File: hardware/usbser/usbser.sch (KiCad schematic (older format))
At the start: 18 parts, among them J2 STM32WORLD_BASE, U1 XC6206P332MR, U2 CP2102N

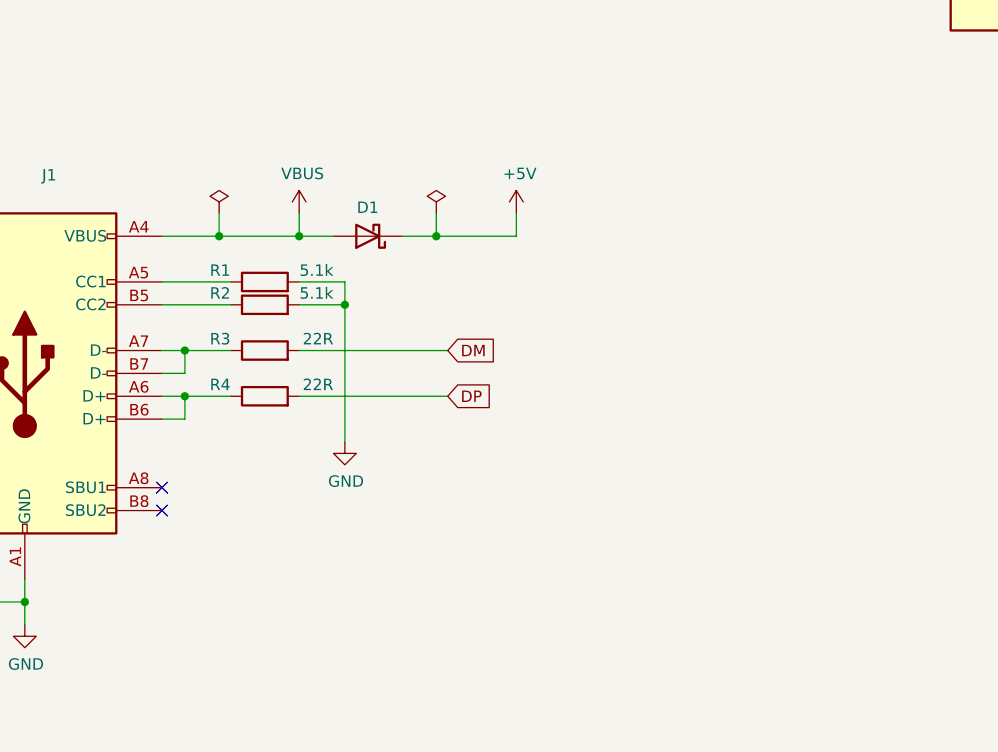
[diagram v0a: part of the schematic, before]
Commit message: Hmmmm
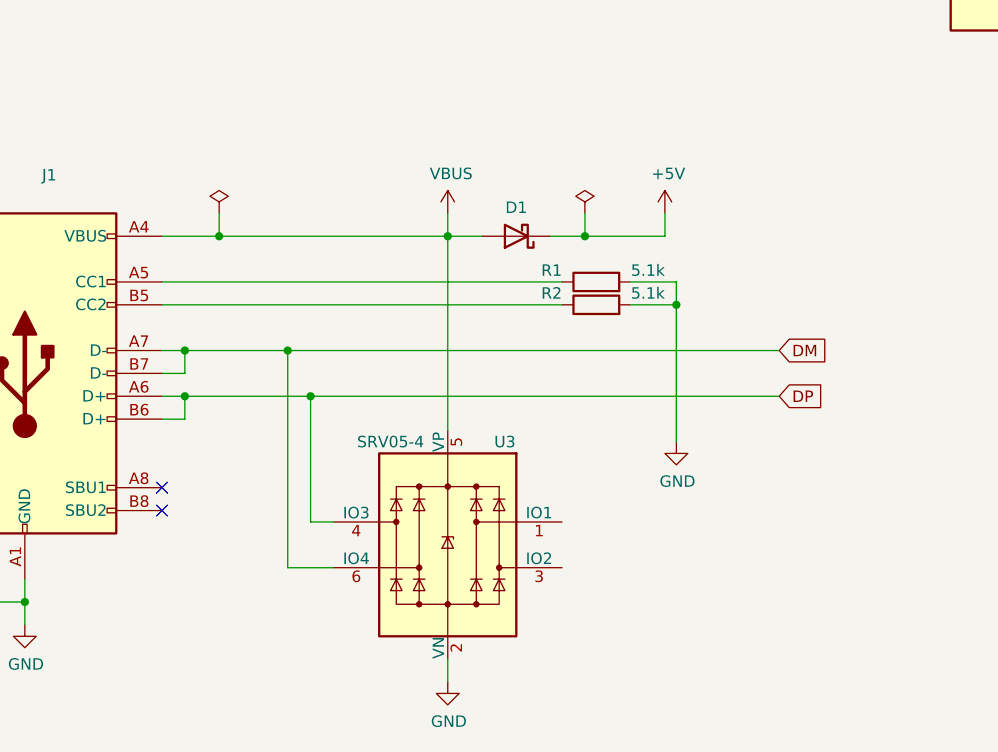
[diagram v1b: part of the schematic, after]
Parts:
- removed R3, R4: 22R, Resistor_SMD:R_0402_1005Metric, symbol Device:R
- added U3: SRV05-4, Package_TO_SOT_SMD:SOT-23-6, symbol Power_Protection:SRV05-4
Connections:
- net DM: now also J1.A7 (D-), J1.B7 (D-), U3.6 (IO4)
- net DP: now also J1.A6 (D+), J1.B6 (D+), U3.4 (IO3)
- net GND: now also U3.2 (VN)
- net VBUS: now also U3.5 (VP)
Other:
- moved on the sheet: D1, R1, R2
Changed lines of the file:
@@
 L Device:D_Schottky D?
 U 1 1 61254E07
-P 2800 5500
+P 3450 5500
 AR Path="/60D07374/61254E07" Ref="D?"  Part="1"
 AR Path="/61254E07" Ref="D1"  Part="1"
-F 0 "D1" H 2800 5375 50  0000 C CNN
-F 1 "~" H 2800 5374 50  0000 C CNN
-F 2 "Diode_SMD:D_SOD-123" H 2800 5500 50  0001 C CNN
-F 3 "~" H 2800 5500 50  0001 C CNN
-F 4 "C8598" H 2800 5500 50  0001 C CNN "LCSC"
-	1    2800 5500
+F 0 "D1" H 3450 5375 50  0000 C CNN
+F 1 "~" H 3450 5374 50  0000 C CNN
+F 2 "Diode_SMD:D_SOD-123" H 3450 5500 50  0001 C CNN
+F 3 "~" H 3450 5500 50  0001 C CNN
+F 4 "C8598" H 3450 5500 50  0001 C CNN "LCSC"
+	1    3450 5500
 	-1   0    0    1
 $EndComp
@@
 Wire Wire Line
 	1900 6000 2000 6000
-Text GLabel 3150 6200 2    50   Input ~ 0
+Text GLabel 4600 6200 2    50   Input ~ 0
 DP
-Text GLabel 3150 6000 2    50   Input ~ 0
+Text GLabel 4600 6000 2    50   Input ~ 0
 DM
 $Comp
 L Device:R R?
 U 1 1 61254E17
-P 2350 5700
+P 3800 5700
 AR Path="/60D07374/61254E17" Ref="R?"  Part="1"
 AR Path="/61254E17" Ref="R1"  Part="1"
-F 0 "R1" V 2400 5850 50  0000 L CNN
-F 1 "5.1k" V 2400 5400 50  0000 L CNN
-F 2 "Resistor_SMD:R_0402_1005Metric" V 2280 5700 50  0001 C CNN
-F 3 "~" H 2350 5700 50  0001 C CNN
-F 4 "C25905" H 2350 5700 50  0001 C CNN "LCSC"
-	1    2350 5700
+F 0 "R1" V 3850 5850 50  0000 L CNN
+F 1 "5.1k" V 3850 5400 50  0000 L CNN
+F 2 "Resistor_SMD:R_0402_1005Metric" V 3730 5700 50  0001 C CNN
+F 3 "~" H 3800 5700 50  0001 C CNN
+F 4 "C25905" H 3800 5700 50  0001 C CNN "LCSC"
+	1    3800 5700
 	0    -1   -1   0
 $EndComp
@@
 L Device:R R?
 U 1 1 61254E2C
-P 2350 5800
+P 3800 5800
 AR Path="/60D07374/61254E2C" Ref="R?"  Part="1"
 AR Path="/61254E2C" Ref="R2"  Part="1"
-F 0 "R2" V 2400 5950 50  0000 L CNN
-F 1 "5.1k" V 2400 5500 50  0000 L CNN
-F 2 "Resistor_SMD:R_0402_1005Metric" V 2280 5800 50  0001 C CNN
-F 3 "~" H 2350 5800 50  0001 C CNN
-F 4 "C25905" H 2350 5800 50  0001 C CNN "LCSC"
-	1    2350 5800
+F 0 "R2" V 3850 5950 50  0000 L CNN
+F 1 "5.1k" V 3850 5500 50  0000 L CNN
+F 2 "Resistor_SMD:R_0402_1005Metric" V 3730 5800 50  0001 C CNN
+F 3 "~" H 3800 5800 50  0001 C CNN
+F 4 "C25905" H 3800 5800 50  0001 C CNN "LCSC"
+	1    3800 5800
 	0    -1   -1   0
 $EndComp
@@
 L power:VBUS #PWR?
 U 1 1 61254E38
-P 2500 5400
+P 3150 5400
 AR Path="/60D07374/61254E38" Ref="#PWR?"  Part="1"
 AR Path="/61254E38" Ref="#PWR0102"  Part="1"
-F 0 "#PWR0102" H 2500 5250 50  0001 C CNN
-F 1 "VBUS" H 2515 5573 50  0000 C CNN
-F 2 "" H 2500 5400 50  0001 C CNN
-F 3 "" H 2500 5400 50  0001 C CNN
-	1    2500 5400
-	1    0    0    -1
-$EndComp
-Wire Wire Line
-	2950 5500 3100 5500
-Wire Wire Line
-	3450 5500 3450 5400
+F 0 "#PWR0102" H 3150 5250 50  0001 C CNN
+F 1 "VBUS" H 3165 5573 50  0000 C CNN
+F 2 "" H 3150 5400 50  0001 C CNN
+F 3 "" H 3150 5400 50  0001 C CNN
+	1    3150 5400
+	1    0    0    -1
+$EndComp
+Wire Wire Line
+	3600 5500 3750 5500
+Wire Wire Line
+	4100 5500 4100 5400
 $Comp
 L power:+5V #PWR?
 U 1 1 61254E40
-P 3450 5400
+P 4100 5400
 AR Path="/60D07374/61254E40" Ref="#PWR?"  Part="1"
 AR Path="/61254E40" Ref="#PWR0103"  Part="1"
-F 0 "#PWR0103" H 3450 5250 50  0001 C CNN
-F 1 "+5V" H 3465 5573 50  0000 C CNN
-F 2 "" H 3450 5400 50  0001 C CNN
-F 3 "" H 3450 5400 50  0001 C CNN
-	1    3450 5400
-	1    0    0    -1
-$EndComp
-Wire Wire Line
-	2500 5400 2500 5500
-Connection ~ 2500 5500
-Wire Wire Line
-	2500 5500 2650 5500
-$Comp
-L Device:R R?
-U 1 1 61254E4A
-P 2350 6000
-AR Path="/60D07374/61254E4A" Ref="R?"  Part="1"
-AR Path="/61254E4A" Ref="R3"  Part="1"
-F 0 "R3" V 2400 6150 50  0000 L CNN
-F 1 "22R" V 2400 5700 50  0000 L CNN
-F 2 "Resistor_SMD:R_0402_1005Metric" V 2280 6000 50  0001 C CNN
-F 3 "~" H 2350 6000 50  0001 C CNN
-F 4 "C25092" H 2350 6000 50  0001 C CNN "LCSC"
-	1    2350 6000
-	0    -1   -1   0
-$EndComp
-$Comp
-L Device:R R?
-U 1 1 61254E51
-P 2350 6200
-AR Path="/60D07374/61254E51" Ref="R?"  Part="1"
-AR Path="/61254E51" Ref="R4"  Part="1"
-F 0 "R4" V 2400 6350 50  0000 L CNN
-F 1 "22R" V 2400 5900 50  0000 L CNN
-F 2 "Resistor_SMD:R_0402_1005Metric" V 2280 6200 50  0001 C CNN
-F 3 "~" H 2350 6200 50  0001 C CNN
-F 4 "C25092" H 2350 6200 50  0001 C CNN "LCSC"
-	1    2350 6200
-	0    -1   -1   0
-$EndComp
-Wire Wire Line
-	3150 6000 2500 6000
-Wire Wire Line
-	3150 6200 2500 6200
-Wire Wire Line
-	2000 6200 2200 6200
-Wire Wire Line
-	2000 6000 2200 6000
+F 0 "#PWR0103" H 4100 5250 50  0001 C CNN
+F 1 "+5V" H 4115 5573 50  0000 C CNN
+F 2 "" H 4100 5400 50  0001 C CNN
+F 3 "" H 4100 5400 50  0001 C CNN
+	1    4100 5400
+	1    0    0    -1
+$EndComp
+Wire Wire Line
+	3150 5400 3150 5500
+Connection ~ 3150 5500
+Wire Wire Line
+	3150 5500 3300 5500
 $Comp
 L power:PWR_FLAG #FLG?
@@
 Connection ~ 2150 5500
 Wire Wire Line
-	2150 5500 2500 5500
+	2150 5500 3150 5500
 NoConn ~ 1900 6600
 NoConn ~ 1900 6700
@@
 L power:PWR_FLAG #FLG?
 U 1 1 61254E66
-P 3100 5400
+P 3750 5400
 AR Path="/60D07374/61254E66" Ref="#FLG?"  Part="1"
 AR Path="/61254E66" Ref="#FLG0102"  Part="1"
-F 0 "#FLG0102" H 3100 5475 50  0001 C CNN
-F 1 "PWR_FLAG" H 3100 5573 50  0001 C CNN
-F 2 "" H 3100 5400 50  0001 C CNN
-F 3 "~" H 3100 5400 50  0001 C CNN
-	1    3100 5400
-	1    0    0    -1
-$EndComp
-Wire Wire Line
-	3100 5400 3100 5500
-Connection ~ 3100 5500
-Wire Wire Line
-	3100 5500 3450 5500
-Wire Wire Line
-	1900 5700 2200 5700
-Wire Wire Line
-	2200 5800 1900 5800
-Wire Wire Line
-	2500 5700 2700 5700
-Wire Wire Line
-	2500 5800 2700 5800
-Wire Wire Line
-	2700 5800 2700 5700
+F 0 "#FLG0102" H 3750 5475 50  0001 C CNN
+F 1 "PWR_FLAG" H 3750 5573 50  0001 C CNN
+F 2 "" H 3750 5400 50  0001 C CNN
+F 3 "~" H 3750 5400 50  0001 C CNN
+	1    3750 5400
+	1    0    0    -1
+$EndComp
+Wire Wire Line
+	3750 5400 3750 5500
+Connection ~ 3750 5500
+Wire Wire Line
+	3750 5500 4100 5500
+Wire Wire Line
+	1900 5700 3650 5700
+Wire Wire Line
+	3650 5800 1900 5800
+Wire Wire Line
+	3950 5700 4150 5700
+Wire Wire Line
+	3950 5800 4150 5800
+Wire Wire Line
+	4150 5800 4150 5700
 $Comp
 L Device:C C?
@@
 L power:GND #PWR?
 U 1 1 6128107B
-P 2700 6400
+P 4150 6400
 AR Path="/60D07374/6128107B" Ref="#PWR?"  Part="1"
 AR Path="/6128107B" Ref="#PWR0109"  Part="1"
-F 0 "#PWR0109" H 2700 6150 50  0001 C CNN
-F 1 "GND" H 2705 6227 50  0000 C CNN
-F 2 "" H 2700 6400 50  0001 C CNN
-F 3 "" H 2700 6400 50  0001 C CNN
-	1    2700 6400
-	1    0    0    -1
-$EndComp
-Wire Wire Line
-	2700 5800 2700 6400
-Connection ~ 2700 5800
+F 0 "#PWR0109" H 4150 6150 50  0001 C CNN
+F 1 "GND" H 4155 6227 50  0000 C CNN
+F 2 "" H 4150 6400 50  0001 C CNN
+F 3 "" H 4150 6400 50  0001 C CNN
+	1    4150 6400
+	1    0    0    -1
+$EndComp
+Wire Wire Line
+	4150 5800 4150 6400
+Connection ~ 4150 5800
 Text GLabel 5150 2800 0    50   Input ~ 0
 DP
@@
 Wire Wire Line
 	10000 5100 9900 5100
+$Comp
+L Power_Protection:SRV05-4 U3
+U 1 1 60D4D417
+P 3150 6850
+F 0 "U3" H 2900 7300 50  0000 C CNN
+F 1 "SRV05-4" H 3400 7300 50  0000 C CNN
+F 2 "Package_TO_SOT_SMD:SOT-23-6" H 3850 6400 50  0001 C CNN
+F 3 "http://www.onsemi.com/pub/Collateral/SRV05-4-D.PDF" H 3150 6850 50  0001 C CNN
+F 4 "C85364" H 3150 6850 50  0001 C CNN "LCSC"
+	1    3150 6850
+	-1   0    0    -1
+$EndComp
+Wire Wire Line
+	2000 6000 2450 6000
+Wire Wire Line
+	2000 6200 2550 6200
+$Comp
+L power:GND #PWR?
+U 1 1 60D5D9D8
+P 3150 7450
+AR Path="/60D07374/60D5D9D8" Ref="#PWR?"  Part="1"
+AR Path="/60D5D9D8" Ref="#PWR0110"  Part="1"
+F 0 "#PWR0110" H 3150 7200 50  0001 C CNN
+F 1 "GND" H 3155 7277 50  0000 C CNN
+F 2 "" H 3150 7450 50  0001 C CNN
+F 3 "" H 3150 7450 50  0001 C CNN
+	1    3150 7450
+	1    0    0    -1
+$EndComp
+Wire Wire Line
+	3150 7450 3150 7350
+Wire Wire Line
+	3150 5500 3150 6350
+Wire Wire Line
+	2650 6750 2550 6750
+Wire Wire Line
+	2550 6750 2550 6200
+Connection ~ 2550 6200
+Wire Wire Line
+	2550 6200 4600 6200
+Wire Wire Line
+	2650 6950 2450 6950
+Wire Wire Line
+	2450 6950 2450 6000
+Connection ~ 2450 6000
+Wire Wire Line
+	2450 6000 4600 6000
 $EndSCHEMATC
